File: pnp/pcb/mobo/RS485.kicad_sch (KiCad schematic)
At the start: 7 parts, among them J22 FEEDERS, U15 MAX3078E

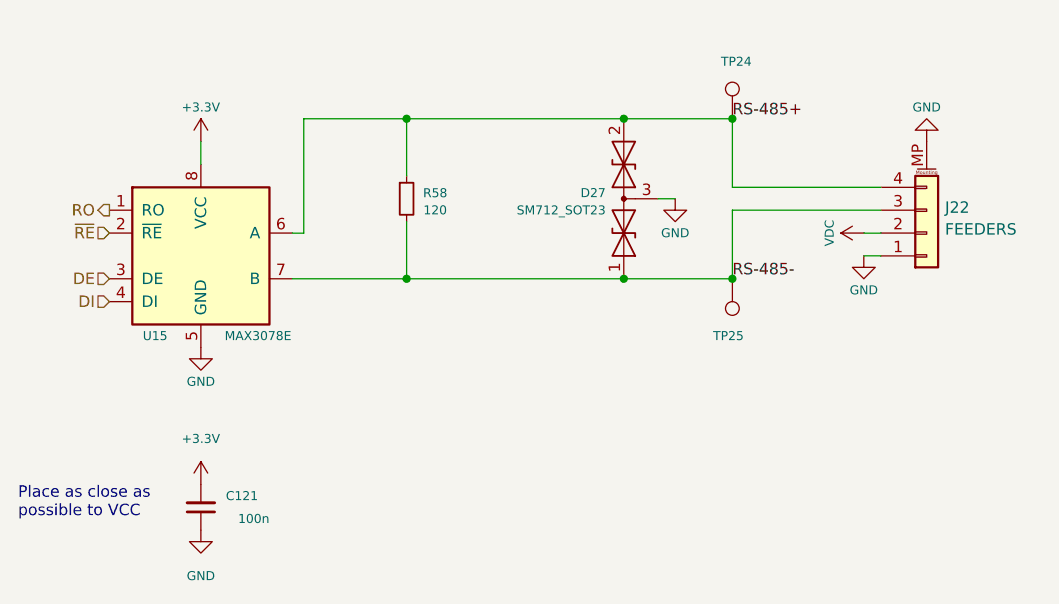
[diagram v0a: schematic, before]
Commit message: Update RS485 to use THVD1400DR with split RC filter termination
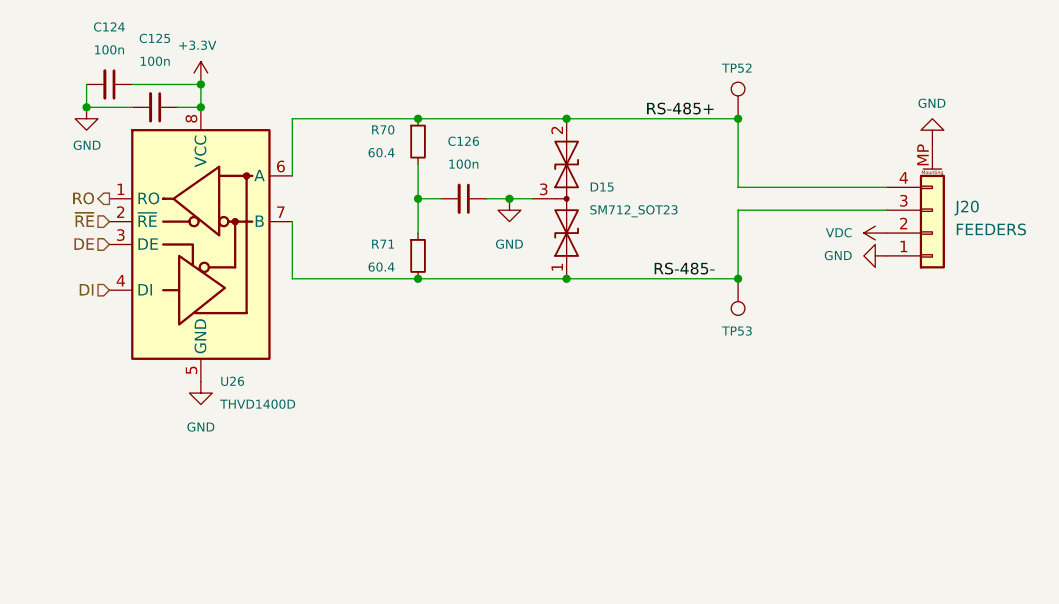
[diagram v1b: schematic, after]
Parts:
- added C124, C126: 100n, Capacitor_SMD:C_0805_2012Metric, symbol Device:C_Small
- added R71: 60.4, Resistor_SMD:R_0805_2012Metric, symbol Device:R_Small
- R70: renamed from R58; value 120 -> 60.4; Digikey 541-120CCT-ND -> 13-RT0805FRE0760R4LCT-ND; JLCPCB C25280 -> C72998; LCSC C25280 -> C72998; Mouser 71-CRCW0805120RFKEA -> 603-RT0805FRE0760R4L
- U26: renamed from U15; value MAX3078E -> THVD1400D; symbol Interface_UART:MAX3078E -> Interface_UART:THVD1400D; Digikey MAX3078EASA+-ND -> 296-THVD1400DRCT-ND; JLCPCB C40031 -> C3235232; LCSC C40031 -> C3235232; Mouser 700-MAX3078EESA -> 595-THVD1400DR
- renumbered C121 to C125, D27 to D15, J22 to J20, TP24 to TP52, TP25 to TP53
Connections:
- net +3.3V: now also C125.1, C124.1; no longer C125.2
- net GND: now also C125.2, C124.2, C126.1; no longer C125.1
- net RS-485-: now also R71.2; no longer R70.2
- new net: C126.2, R70.2, R71.1
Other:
- note removed: "Place as close as possible to VCC"
- moved on the sheet: C125, D15, J20, R70, TP52, TP53
